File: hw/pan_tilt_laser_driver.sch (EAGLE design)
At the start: 37 parts, among them IC2 998-MIC5219-3.0YMM, IC3 FT2232H, IC5 93C46, IC6 998-MIC5219-3.0YMM, X1 798-ZX62RD-AB-5P8, X2 12MHz

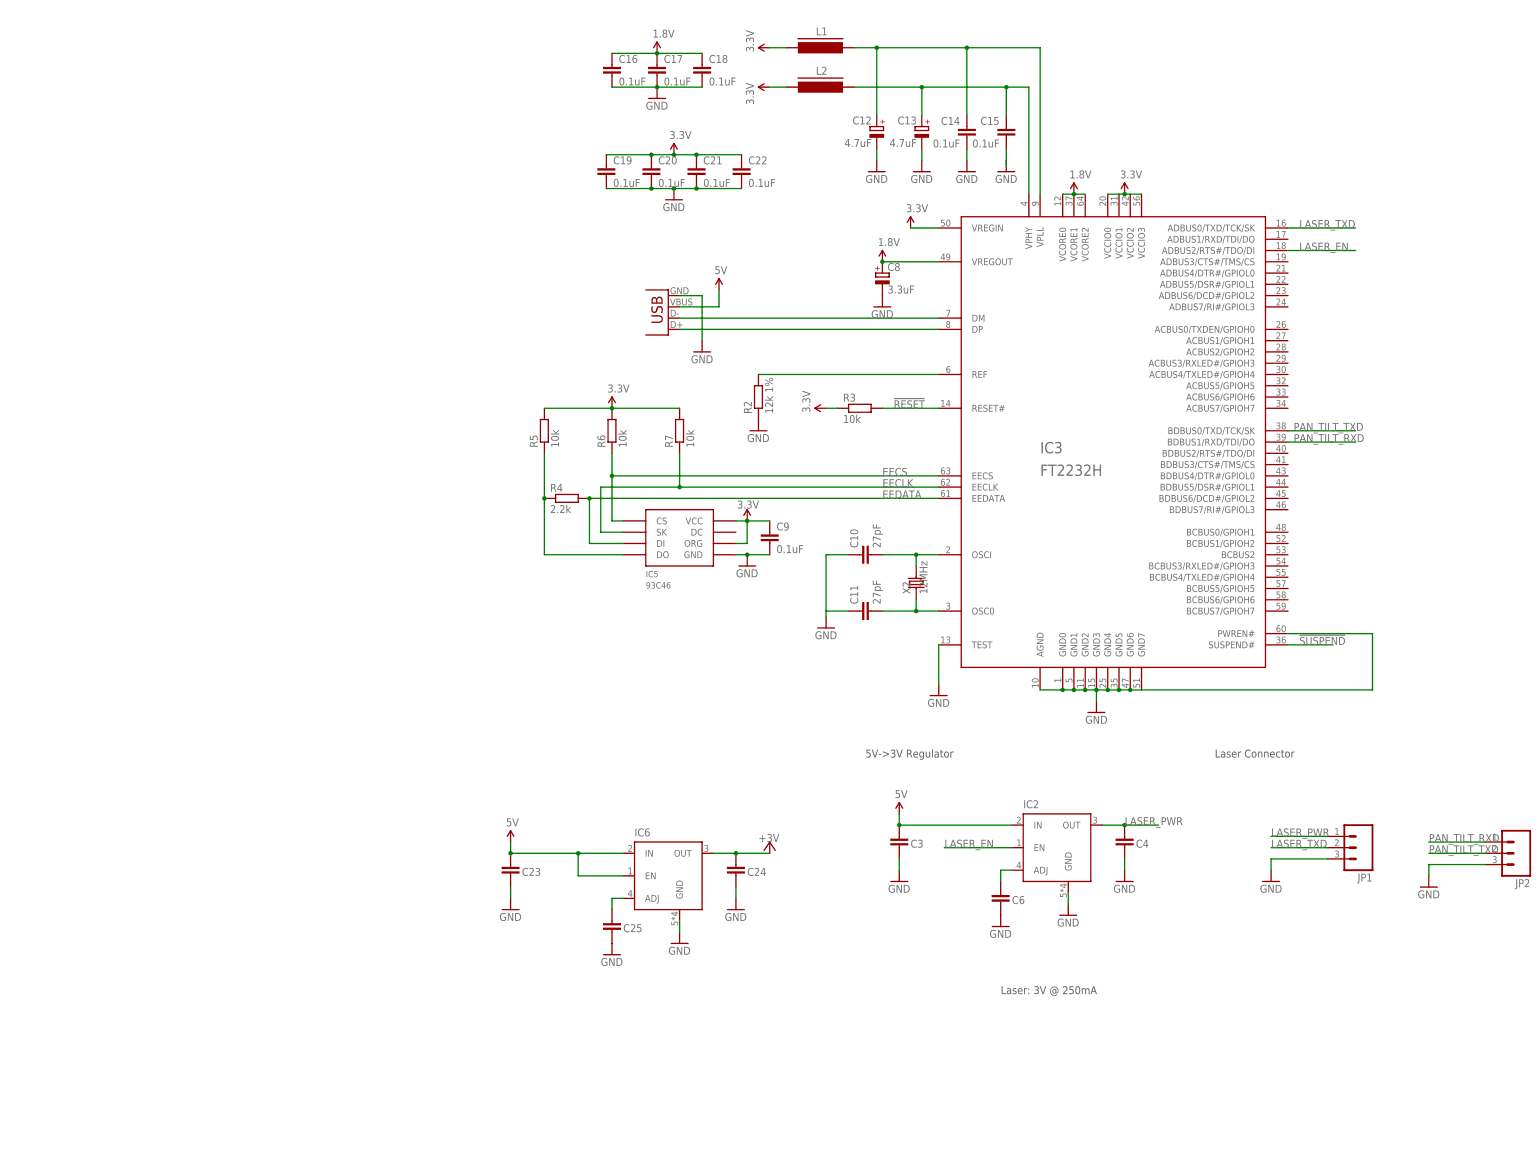
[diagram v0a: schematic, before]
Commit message: Outline replaced, in progress
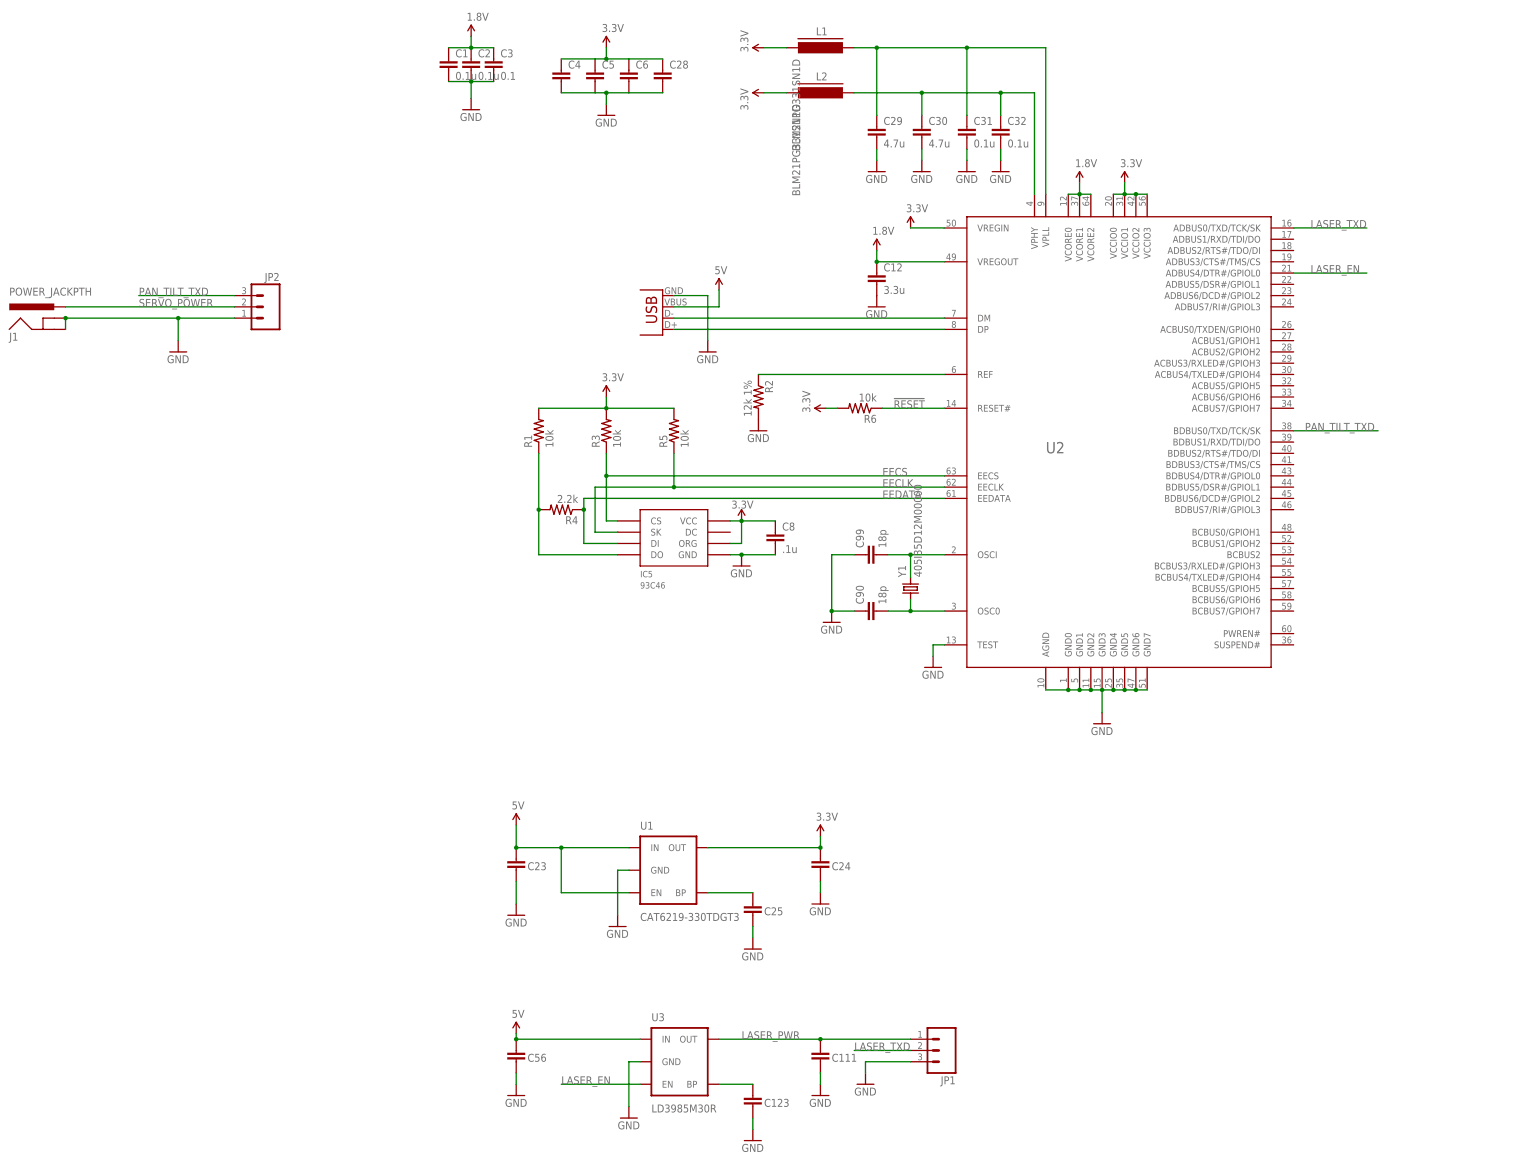
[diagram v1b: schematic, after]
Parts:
- removed C10, C11: 27pF, dp_devices:CAPC805
- removed C13: 4.7uF, dp_devices:CAP_POLSMC_A
- removed C14, C15, C16, C17, C18, C19, C20, C21, C22, C9: 0.1uF, dp_devices:CAPC805
- removed IC2, IC6: 998-MIC5219-3.0YMM, v-reg-micrel:MIC5219BMM
- removed IC3: FT2232H, DP-EagleLibrary:FT2232H
- removed R7: 10k, dp_devices:RESISTORR805R805
- removed X2: 12MHz, dp_devices:CRYSTAL_212M_
- added C1, C2, C31, C32: 0.1u, rcl:C-EUC0603K
- added C111, C56: C1608X5R1C106M080AB, SparkFun-Passives:CAP0603-CAP
- added C123: VJ0603A471KXQPW1BC, SparkFun-Passives:CAP0603-CAP
- added C28, C5: (no value), rcl:C-EUC0603K
- added C29, C30: 4.7u, rcl:C-EUC0603K
- added C90, C99: 18p, rcl:C-EUC0603K
- added J1: POWER_JACKPTH, SparkFun-Connectors:POWER_JACKPTH
- added R1: 10k, rcl:R-US_R0603
- added U1: CAT6219-330TDGT3, SparkFun-PowerIC:V_REG_MIC52195V
- added U2: (no value), torpedo:FT2232H
- added U3: LD3985M30R, SparkFun-PowerIC:V_REG_MIC52195V
- added Y1: 405I35D12M00000, SparkFun-FreqCtrl:CRYSTAL5X3
- C12: value 4.7uF -> 3.3u; device dp_devices:CAP_POLSMC_A -> rcl:C-EUC0603K
- C3: value C1608X5R1C106M080AB -> 0.1; device SparkFun-Passives:CAP0603-CAP -> rcl:C-EUC0603K
- C4: value C1608X5R1C106M080AB -> (none); device SparkFun-Passives:CAP0603-CAP -> rcl:C-EUC0603K
- C6: value VJ0603A471KXQPW1BC -> (none); device SparkFun-Passives:CAP0603-CAP -> rcl:C-EUC0603K
- C8: value 3.3uF -> .1u; device dp_devices:CAP_POLSMC_A -> rcl:C-EUC0603K
- JP2: value 651-5442251 -> (none); device SparkFun-Connectors:M03SCREW -> torpedo:M0322-03-5035
- L1, L2: value (none) -> BLM21PG331SN1D
- R2, R3, R4, R5, R6: device dp_devices:RESISTORR805R805 -> rcl:R-US_R0603
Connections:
- removed net !SUSPEND: IC3.SUSPEND#
- removed net +3V3: C24.1, IC6.OUT
- removed net N$2: C6.1, IC2.ADJ
- removed net PAN_TILT_RXD: IC3.BDBUS1/RXD/TDI/DO, JP2.1
- new net N$8: C25.1, U1.BP
- new net SERVO_POWER: J1.PWR, JP2.2
- net !RESET: now also R6.1, U2.RESET#; no longer IC3.RESET#, R3.2
- net 1.8V: now also C1.1, C12.1, C2.1, C3.1, U2.VCORE0, U2.VCORE1, U2.VCORE2, U2.VREGOUT; no longer C16.1, C17.1, C18.1, C8.+, IC3.VCORE0, IC3.VCORE1, IC3.VCORE2, IC3.VREGOUT
- net 3.3V: now also C24.1, C28.1, C4.1, C5.1, C6.1, C8.1, R1.2, R3.2, U1.OUT, U2.VCCIO0, U2.VCCIO1, U2.VCCIO2, U2.VCCIO3, U2.VREGIN; no longer C19.1, C20.1, C21.1, C22.1, C9.1, IC3.VCCIO0, IC3.VCCIO1, IC3.VCCIO2, IC3.VCCIO3, IC3.VREGIN, R3.1, R7.2
- net 5V: now also C56.1, U1.EN, U1.IN, U3.IN; no longer C3.1, IC2.IN, IC6.EN, IC6.IN
- net EECLK: now also R5.1, U2.EECLK; no longer IC3.EECLK, R7.1
- net EECS: now also R3.1, U2.EECS; no longer IC3.EECS, R6.1
- net EEDATA: now also R4.1, U2.EEDATA; no longer IC3.EEDATA, R4.2
- net GND: now also C1.2, C111.2, C12.2, C123.2, C2.2, C28.2, C29.2, C30.2, C31.2, C32.2, C5.2, C56.2, C8.2, C90.1, C99.1, J1.GND, J1.GNDBREAK, JP2.1, R2.2, U1.GND, U2.AGND, U2.GND0, U2.GND1, U2.GND2, U2.GND3, U2.GND4, U2.GND5, U2.GND6, U2.GND7, U2.TEST, U3.GND; no longer C10.1, C11.1, C12.-, C13.-, C14.2, C15.2, C16.2, C17.2, C18.2, C19.2, C20.2, C21.2, C22.2, C8.-, C9.2, IC2.GND, IC3.AGND, IC3.GND0, IC3.GND1, IC3.GND2, IC3.GND3, IC3.GND4, IC3.GND5, IC3.GND6, IC3.GND7, IC3.PWREN#, IC3.TEST, IC6.GND, JP2.3, R2.1
- net LASER_EN: now also U2.ADBUS4/DTR#/GPIOL0, U3.EN; no longer IC2.EN, IC3.ADBUS2/RTS#/TDO/DI
- net LASER_PWR: now also C111.1, U3.OUT; no longer C4.1, IC2.OUT
- net LASER_TXD: now also U2.ADBUS0/TXD/TCK/SK; no longer IC3.ADBUS0/TXD/TCK/SK
- net N$1: now also C123.1, U3.BP; no longer C25.1, IC6.ADJ
- net N$10: now also C90.2, U2.OSC0, Y1.1; no longer C11.2, IC3.OSC0, X2.X1
- net N$3: now also U2.DM; no longer IC3.DM
- net N$4: now also R2.1, U2.REF; no longer IC3.REF, R2.2
- net N$45: now also R1.1, R4.2; no longer R4.1, R5.1
- net N$5: now also U2.DP; no longer IC3.DP
- net N$6: now also C29.1, C31.1, U2.VPLL; no longer C12.+, C14.1, IC3.VPLL
- net N$7: now also C99.2, U2.OSCI, Y1.2; no longer C10.2, IC3.OSCI, X2.X2
- net N$9: now also C30.1, C32.1, U2.VPHY; no longer C13.+, C15.1, IC3.VPHY
- net PAN_TILT_TXD: now also JP2.3, U2.BDBUS0/TXD/TCK/SK; no longer IC3.BDBUS0/TXD/TCK/SK, JP2.2
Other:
- note removed: "5V->3V Regulator"
- note removed: "Laser Connector"
- note removed: "Laser: 3V @ 250mA"
- moved on the sheet: C23, C24, C25, C3, C4, C6, IC5, JP1, JP2, L2
